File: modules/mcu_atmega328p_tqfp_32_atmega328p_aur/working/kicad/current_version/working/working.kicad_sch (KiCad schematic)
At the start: 1 part, among them J1 itq32at328_electronic_ic_tqfp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

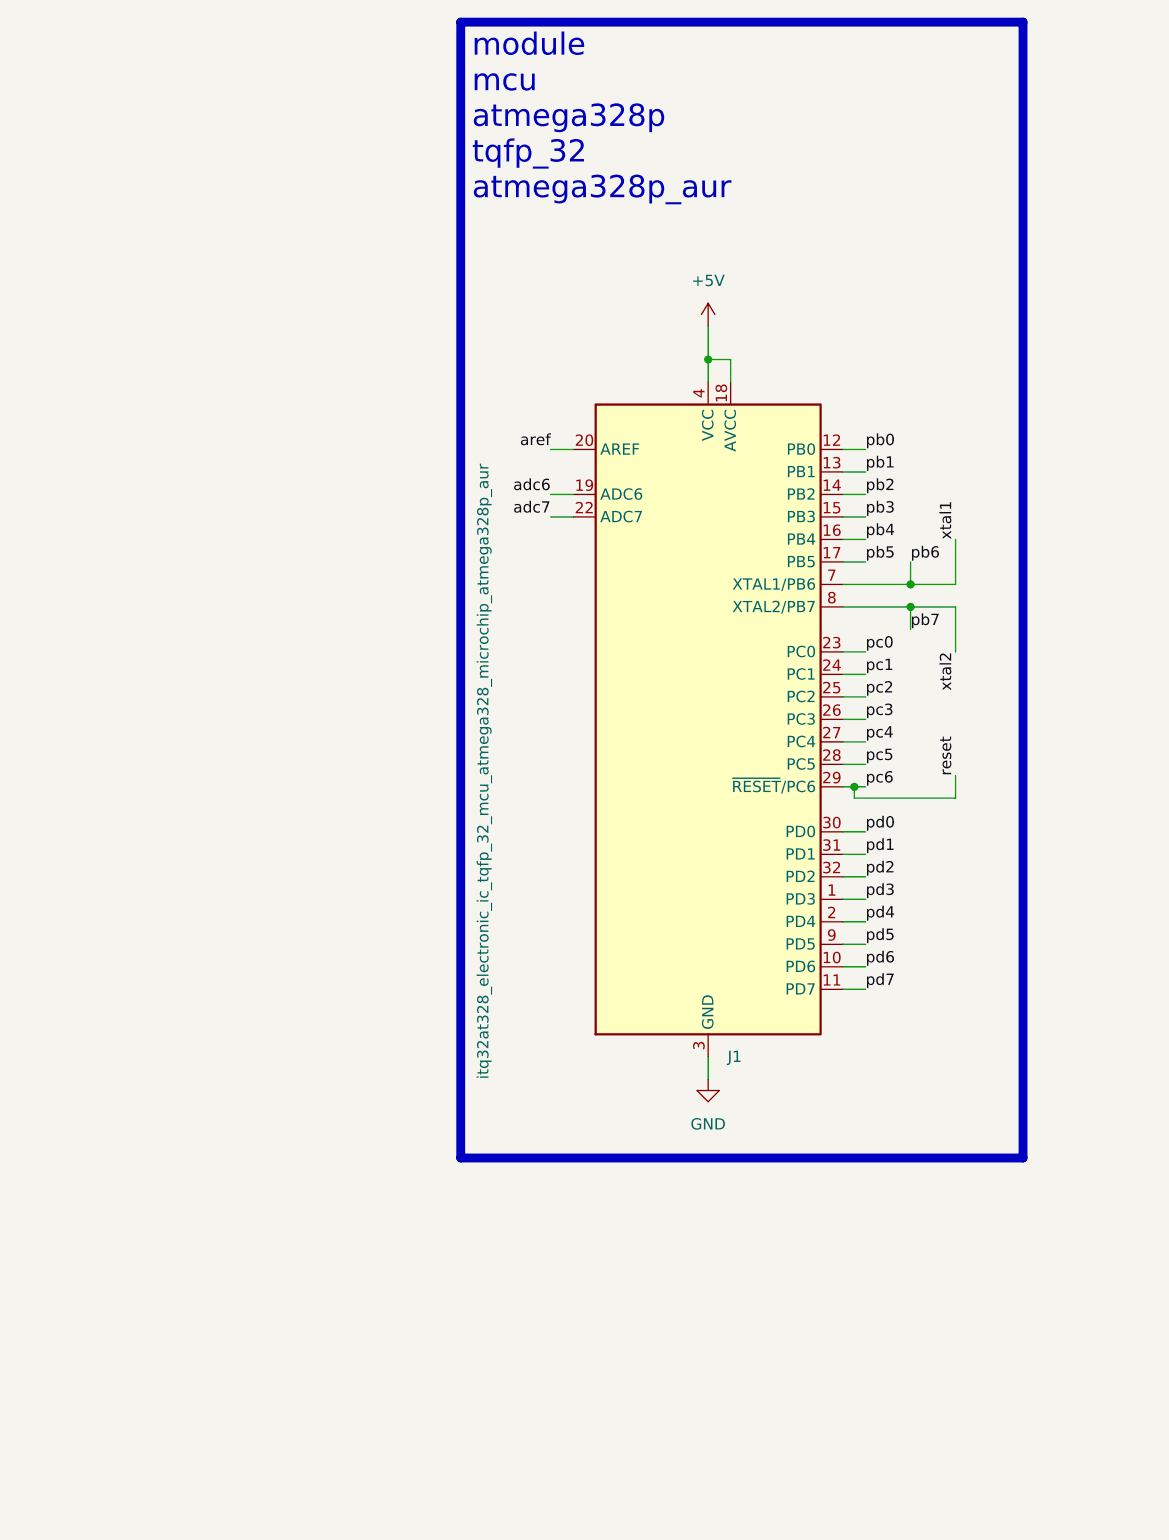
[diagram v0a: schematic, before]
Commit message: workings
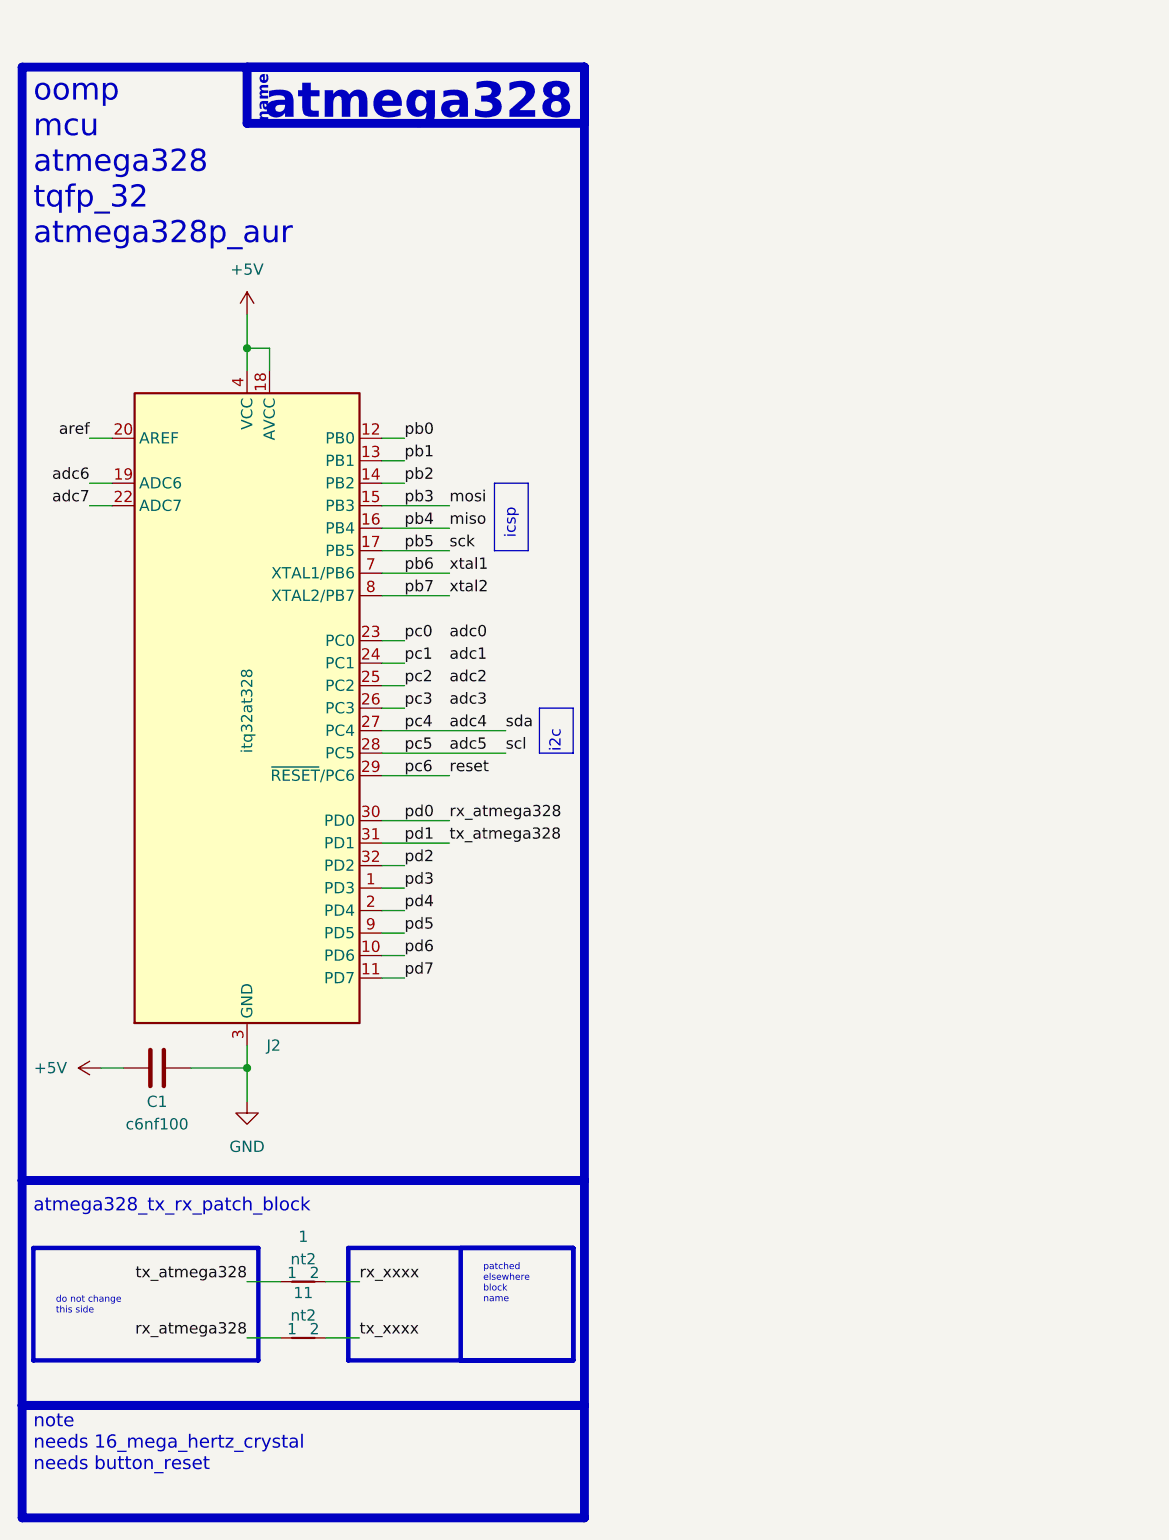
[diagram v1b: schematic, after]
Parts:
- removed J1: itq32at328_electronic_ic_tqfp_32_mcu_atmega328_mi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, itq32at328_electronic_ic_tqfp_32_mcu_atmega328_microchip_atmega328p_aur, symbol oomlout_oomp_part_symbols:itq32at328_electronic_ic_tqfp_32_mcu_atmega328_microc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
- added 1, 11: nt2, nt2_electronic_nettie_2_nets_smd, symbol oomlout_oomp_part_symbols:nt2_electronic_nettie_2_nets_smd
- added C1: c6nf100, c6nf100_electronic_capacitor_0603_100_nano_farad, symbol oomlout_oomp_part_symbols:c6nf100_electronic_capacitor_0603_100_nano_farad
- added J2: itq32at328, itq32at328_electronic_ic_tqfp_32_mcu_atmega328_microchip_atmega328p_aur, symbol oomlout_oomp_part_symbols:itq32at328_electronic_ic_tqfp_32_mcu_atmega328_microc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
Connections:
- net +5V: now also C1.1, J2.18 (AVCC), J2.4 (VCC), J2.6 (VCC)
- net GND: now also C1.2, J2.21 (GND), J2.3 (GND), J2.5 (GND)
- net adc6: now also J2.19 (ADC6)
- net adc7: now also J2.22 (ADC7)
- net aref: now also J2.20 (AREF)
- net pb0: now also J2.12 (PB0)
- net pb1: now also J2.13 (PB1)
- net pb2: now also J2.14 (PB2)
- net pb5: now also J2.17 (PB5)
- net pb6: now also J2.7 (XTAL1/PB6)
- net pb7: now also J2.8 (XTAL2/PB7)
- net pc0: now also J2.23 (PC0)
- net pc1: now also J2.24 (PC1)
- net pc2: now also J2.25 (PC2)
- net pc3: now also J2.26 (PC3)
- net pc6: now also J2.29 (~{RESET}/PC6)
- net pd0: now also 11.1, J2.30 (PD0)
- net pd1: now also 1.1, J2.31 (PD1)
- net pd2: now also J2.32 (PD2)
- net pd3: now also J2.1 (PD3)
- net pd4: now also J2.2 (PD4)
- net pd5: now also J2.9 (PD5)
- net pd6: now also J2.10 (PD6)
- net pd7: now also J2.11 (PD7)
- new net adc4: J2.27 (PC4)
- new net adc5: J2.28 (PC5)
- new net miso: J2.16 (PB4)
- new net mosi: J2.15 (PB3)
- new net rx_xxxx: 1.2
- new net tx_xxxx: 11.2
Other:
- note added: "atmega328"
- note added: "atmega328_tx_rx_patch_block"
- note added: "do not change this side"
- note added: "i2c"
- note added: "icsp"
- note added: "name"
- note added: "note needs 16_mega_hertz_crystal needs button_reset"
- note added: "oomp mcu atmega328 tqfp_32 atmega328p_aur"
- note added: "patched elsewhere block name"
- note removed: "module mcu atmega328p tqfp_32 atmega328p_aur"

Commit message: gitignore update mainly and update
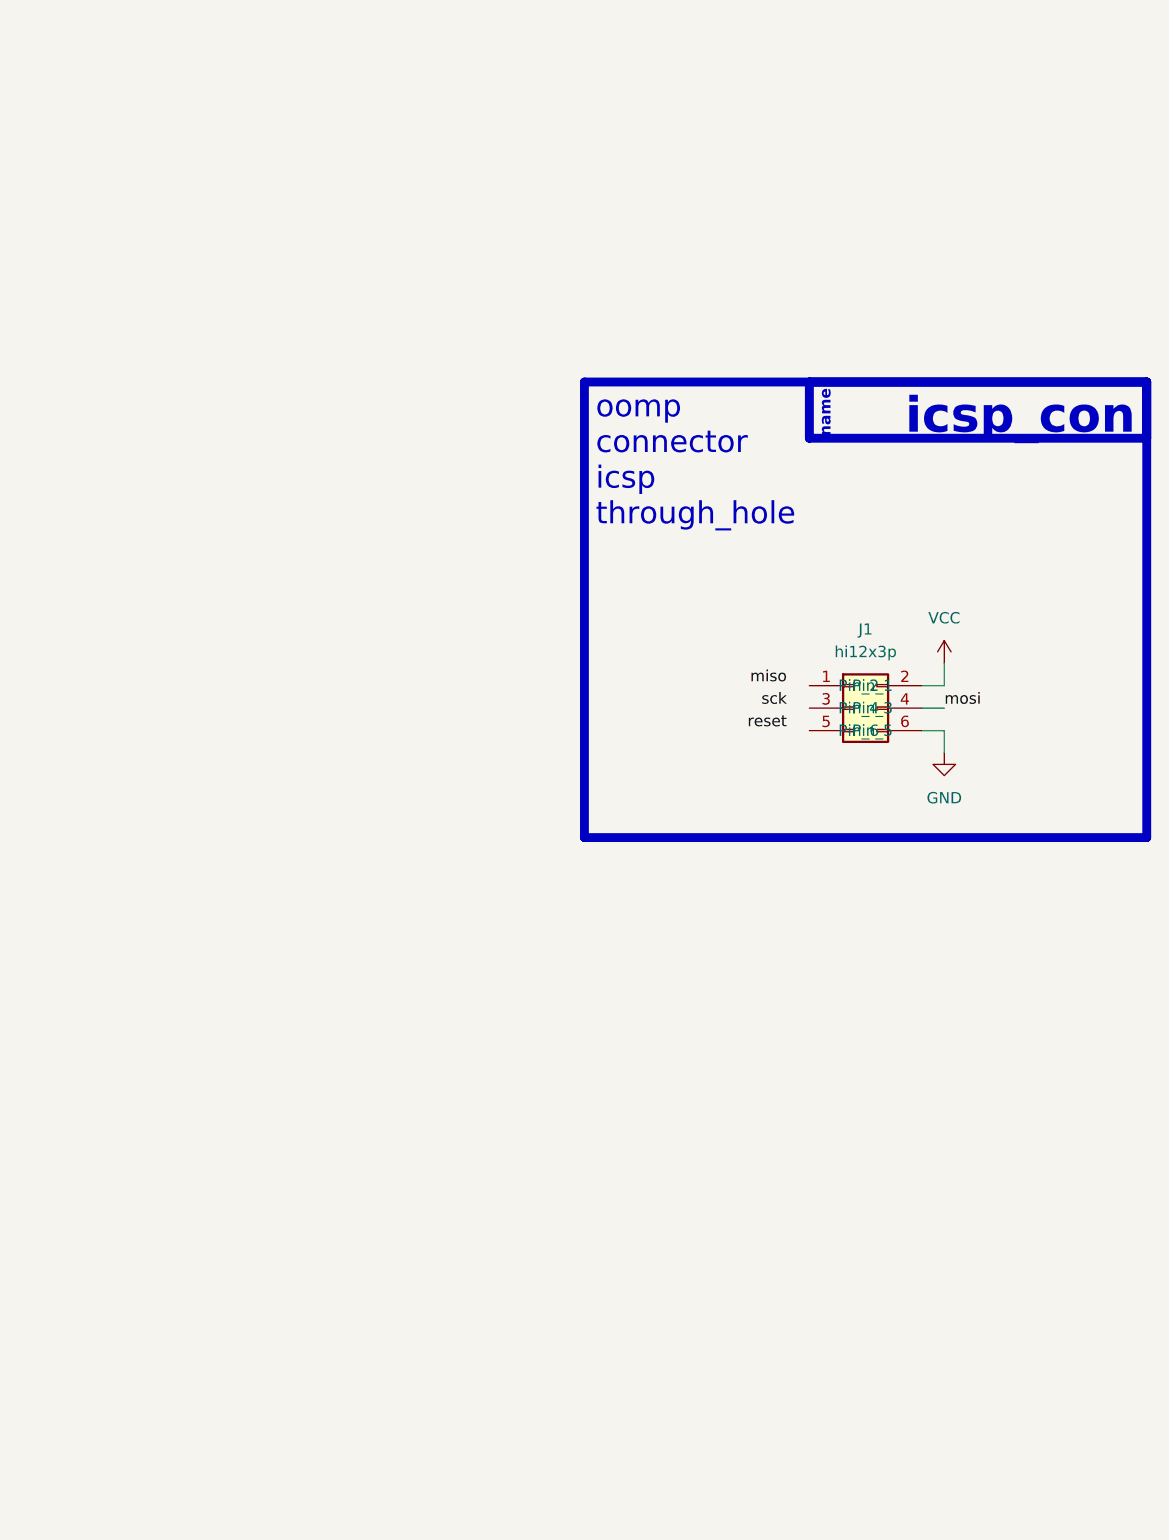
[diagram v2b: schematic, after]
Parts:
- removed 1, 11: nt2, nt2_electronic_nettie_2_nets_smd, symbol oomlout_oomp_part_symbols:nt2_electronic_nettie_2_nets_smd
- removed C1: c6nf100, c6nf100_electronic_capacitor_0603_100_nano_farad, symbol oomlout_oomp_part_symbols:c6nf100_electronic_capacitor_0603_100_nano_farad
- removed J2: itq32at328, itq32at328_electronic_ic_tqfp_32_mcu_atmega328_microchip_atmega328p_aur, symbol oomlout_oomp_part_symbols:itq32at328_electronic_ic_tqfp_32_mcu_atmega328_microc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
- added J1: hi12x3p, hi12x3p_electronic_header_2d54_mm_dual_row_2x3_dual_row_6_pin, symbol oomlout_oomp_part_symbols:hi12x3p_electronic_header_2d54_mm_dual_row_2x3_dual_r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
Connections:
- net GND: now also J1.6 (Pin_6)
- net mosi: now also J1.4 (Pin_4)
- new net VCC: J1.2 (Pin_2)
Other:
- note added: "icsp_con"
- note added: "oomp connector icsp through_hole"
- note removed: "atmega328"
- note removed: "atmega328_tx_rx_patch_block"
- note removed: "do not change this side"
- note removed: "i2c"
- note removed: "icsp"
- note removed: "note needs 16_mega_hertz_crystal needs button_reset"
- note removed: "oomp mcu atmega328 tqfp_32 atmega328p_aur"
- note removed: "patched elsewhere block name"

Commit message: a few module workings
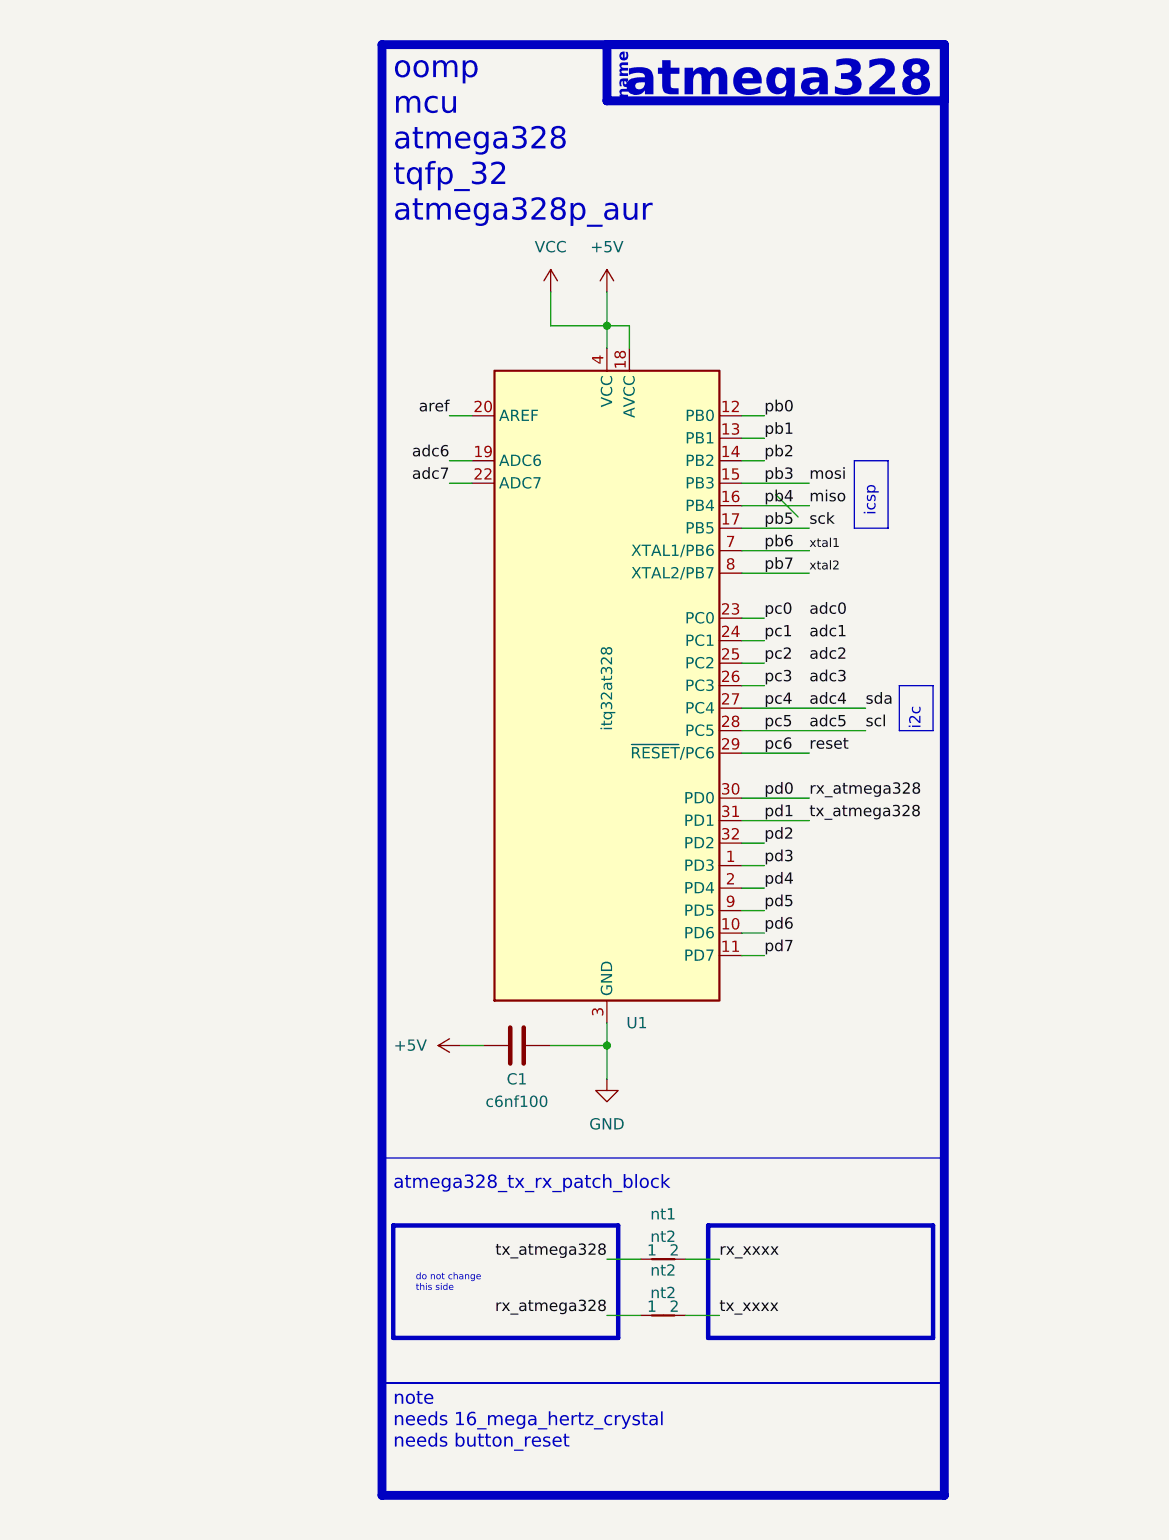
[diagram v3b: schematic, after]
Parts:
- removed J1: hi12x3p, hi12x3p_electronic_header_2d54_mm_dual_row_2x3_dual_row_6_pin, symbol oomlout_oomp_part_symbols:hi12x3p_electronic_header_2d54_mm_dual_row_2x3_dual_r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
- added C1: c6nf100, oomlout_oomp_part_kicad_footprints:c6nf100_electronic_capacitor_0603_100_nano_farad, symbol oomlout_oomp_part_symbols:c6nf100_electronic_capacitor_0603_100_nano_farad
- added U1: itq32at328, oomlout_oomp_part_kicad_footprints:itq32at328_electronic_ic_tqfp_32_mcu_atmega328_microchip_atmega328p_aur, symbol oomlout_oomp_part_symbols:itq32at328_electronic_ic_tqfp_32_mcu_atmega328_microc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
- added nt1, nt2: nt2, oomlout_oomp_part_kicad_footprints:nt2_electronic_nettie_2_nets_smd, symbol oomlout_oomp_part_symbols:nt2_electronic_nettie_2_nets_smd
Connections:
- net GND: now also C1.2, U1.21 (GND), U1.3 (GND), U1.5 (GND)
- net miso: now also U1.16 (PB4)
- net mosi: now also U1.15 (PB3)
- new net +5V: C1.1, U1.18 (AVCC), U1.4 (VCC), U1.6 (VCC)
- new net adc4: U1.27 (PC4)
- new net adc5: U1.28 (PC5)
- new net adc6: U1.19 (ADC6)
- new net adc7: U1.22 (ADC7)
- new net aref: U1.20 (AREF)
- new net pb0: U1.12 (PB0)
- new net pb1: U1.13 (PB1)
- new net pb2: U1.14 (PB2)
- new net pb5: U1.17 (PB5)
- new net pb6: U1.7 (XTAL1/PB6)
- new net pb7: U1.8 (XTAL2/PB7)
- new net pc0: U1.23 (PC0)
- new net pc1: U1.24 (PC1)
- new net pc2: U1.25 (PC2)
- new net pc3: U1.26 (PC3)
- new net pc6: U1.29 (~{RESET}/PC6)
- new net pd0: U1.30 (PD0), nt2.1
- new net pd1: U1.31 (PD1), nt1.1
- new net pd2: U1.32 (PD2)
- new net pd3: U1.1 (PD3)
- new net pd4: U1.2 (PD4)
- new net pd5: U1.9 (PD5)
- new net pd6: U1.10 (PD6)
- new net pd7: U1.11 (PD7)
- new net rx_xxxx: nt1.2
- new net tx_xxxx: nt2.2
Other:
- note added: "atmega328"
- note added: "atmega328_tx_rx_patch_block"
- note added: "do not change this side"
- note added: "i2c"
- note added: "icsp"
- note added: "note needs 16_mega_hertz_crystal needs button_reset"
- note added: "oomp mcu atmega328 tqfp_32 atmega328p_aur"
- note removed: "icsp_con"
- note removed: "oomp connector icsp through_hole"
